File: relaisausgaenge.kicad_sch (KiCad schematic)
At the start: 9 parts, among them K1 TIANBO-HJR-4102-L, K2 TIANBO-HJR-4102-L, K3 TIANBO-HJR-4102-L, U6 ULN2004A

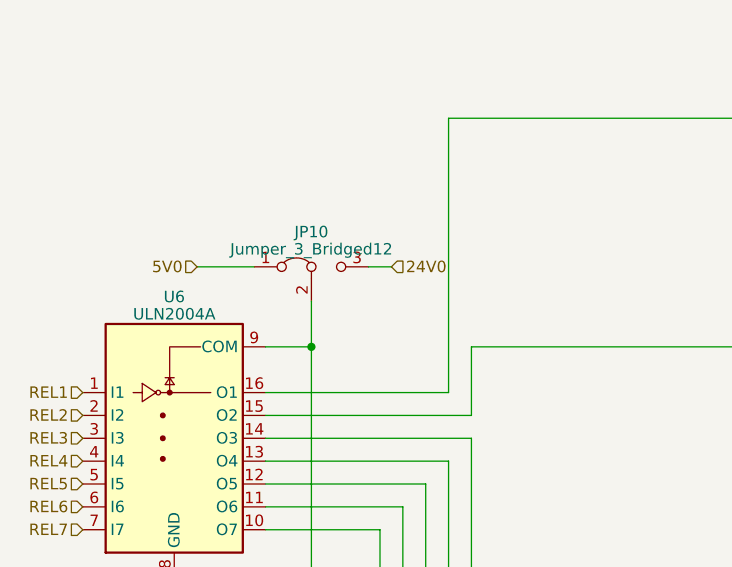
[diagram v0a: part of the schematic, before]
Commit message: placing2
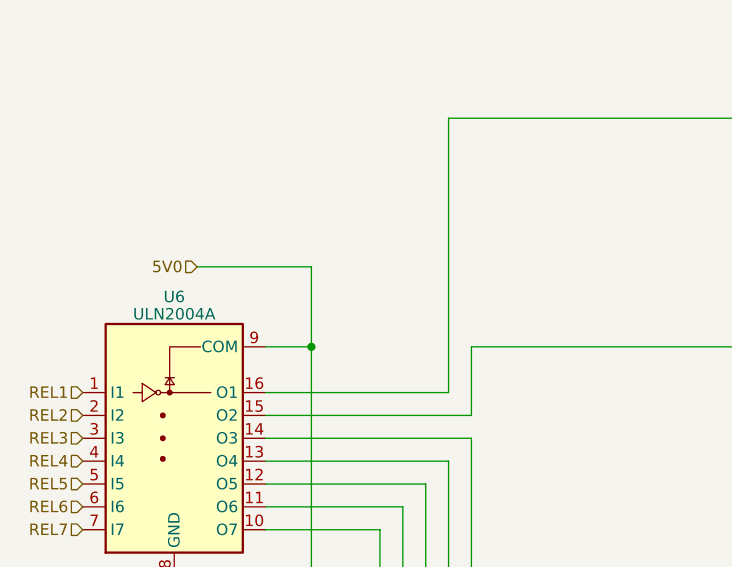
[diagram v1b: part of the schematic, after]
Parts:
- removed JP10: Jumper_3_Bridged12, Connector_PinHeader_2.54mm:PinHeader_1x03_P2.54mm_Vertical, symbol Jumper:Jumper_3_Bridged12
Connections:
- net 5V0: now also EXT_REL_CON1.1 (Pin_1), K1.8, K2.8, K3.8, U6.9 (COM)
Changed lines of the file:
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@@
     (stroke (width 0) (type default))
   )
-  (wire (pts (xy 91.44 74.93) (xy 91.44 80.01))
+  (wire (pts (xy 91.44 71.12) (xy 91.44 80.01))
     (stroke (width 0) (type default))
   )
@@
     (stroke (width 0) (type default))
   )
-  (wire (pts (xy 78.74 71.12) (xy 85.09 71.12))
+  (wire (pts (xy 78.74 71.12) (xy 91.44 71.12))
     (stroke (width 0) (type default))
   )
@@
     (stroke (width 0) (type default))
   )
-  (wire (pts (xy 97.79 71.12) (xy 100.33 71.12))
-    (stroke (width 0) (type default))
-  )
   (wire (pts (xy 106.68 54.61) (xy 146.05 54.61))
     (stroke (width 0) (type default))
@@
   (wire (pts (xy 171.45 67.31) (xy 175.26 67.31))
     (stroke (width 0) (type default))
-  )
-  (hierarchical_label "24V0" (shape input) (at 100.33 71.12 0) (fields_autoplaced)
-    (effects (font (size 1.27 1.27)) (justify left))
   )
   (hierarchical_label "REL2" (shape input) (at 66.04 87.63 180) (fields_autoplaced)
@@
         )
       )
-    )
-  )
-  (symbol (lib_id "Jumper:Jumper_3_Bridged12") (at 91.44 71.12 0) (unit 1)
-    (in_bom yes) (on_board yes) (dnp no) (fields_autoplaced)
-    (property "Reference" "JP10" (at 91.44 67.2459 0)
-      (effects (font (size 1.27 1.27)))
-    )
-    (property "Value" "Jumper_3_Bridged12" (at 91.44 69.1669 0)
-      (effects (font (size 1.27 1.27)))
-    )
-    (property "Footprint" "Connector_PinHeader_2.54mm:PinHeader_1x03_P2.54mm_Vertical" (at 91.44 71.12 0)
-      (effects (font (size 1.27 1.27)) hide)
-    )
-    (property "Datasheet" "~" (at 91.44 71.12 0)
-      (effects (font (size 1.27 1.27)) hide)
-    )
-    (pin "1")
-    (pin "2")
-    (pin "3")
-    (instances
-      (project "rollo control"
-        (path "/7fd4875b-e2b3-49e9-a377-320ee6c6aef7/42cd8867-79f6-4c26-8217-42f6d2cc80dc"
-          (reference "JP10") (unit 1)
-        )
-        (path "/7fd4875b-e2b3-49e9-a377-320ee6c6aef7/f84d4e41-04bc-49f0-bae3-d4cb51e0b9a0"
-          (reference "JP7") (unit 1)
-        )
-      )

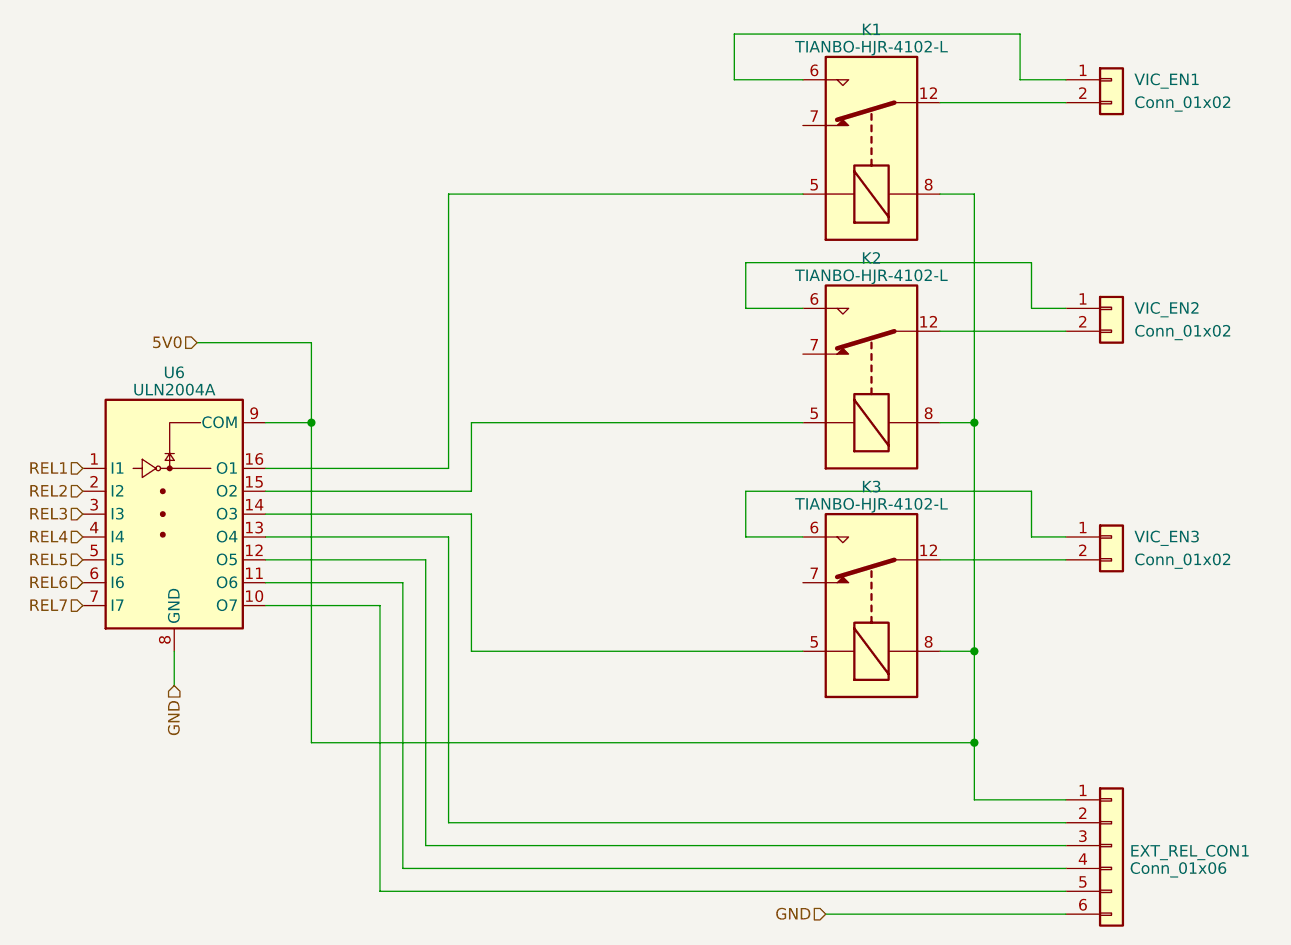
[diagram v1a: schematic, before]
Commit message: gsdfg
dyfg
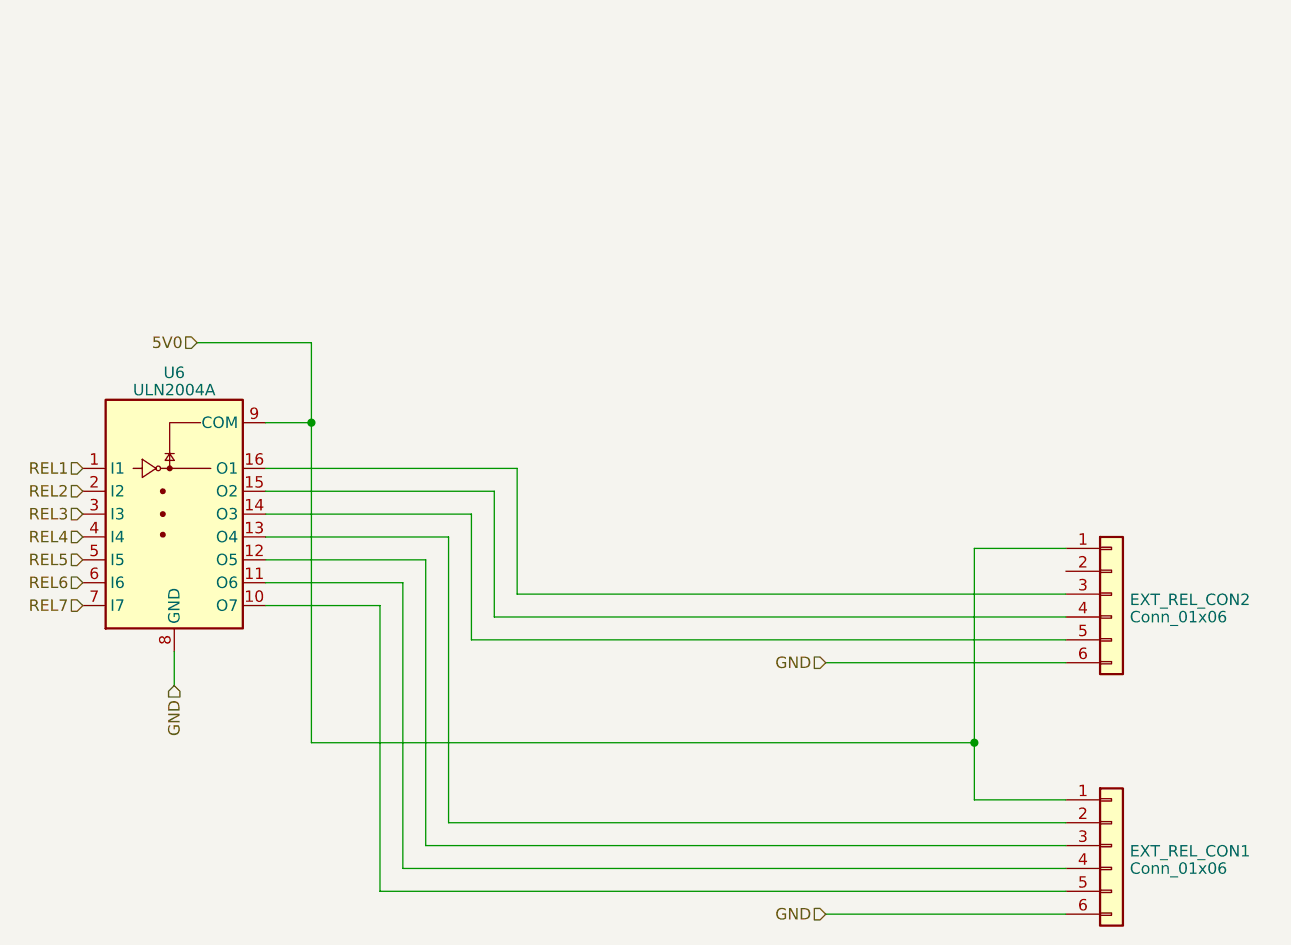
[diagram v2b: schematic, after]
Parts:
- removed K1, K2, K3: TIANBO-HJR-4102-L, Relay_THT:Relay_SPDT_HJR-4102, symbol Relay:TIANBO-HJR-4102-L
- removed VIC_EN1, VIC_EN2, VIC_EN3: Conn_01x02, Connector_Phoenix_MC:PhoenixContact_MC_1,5_2-G-3.5_1x02_P3.50mm_Horizontal, symbol Connector_Generic:Conn_01x02
- added EXT_REL_CON2: Conn_01x06, Connector_JST:JST_XH_B5B-XH-A_1x05_P2.50mm_Vertical, symbol Connector_Generic:Conn_01x06
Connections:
- net 5V0: now also EXT_REL_CON2.1 (Pin_1)
- net GND: now also EXT_REL_CON2.6 (Pin_6)
- net at U6.14 (O3): now also EXT_REL_CON2.5 (Pin_5)
- net at U6.15 (O2): now also EXT_REL_CON2.4 (Pin_4)
- net at U6.16 (O1): now also EXT_REL_CON2.3 (Pin_3)
